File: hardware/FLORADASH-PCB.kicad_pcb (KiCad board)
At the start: 4 copper layers, 141.4 x 50.8 mm, 96 parts, among them IC1 LM66200DRLR, J1 USB_C_Receptacle_USB2.0_16P, J2 Conn_01x04_Pin, J3 Conn_02x04_Top_Bottom, Q1 FS8205, Q2 FS8205, SW1 SW_Push, SW2 SW_Push, U1 TP4056-42-ESOP8, U2 USBLC6-2SC6, U3 DW01A, U4 MT3420SP, U5 MAX17048G_T10, U6 DHT11, U7 CY8CMBR3102, U8 ESP32-C3-WROOM-02, U9 USBLC6-2SC6

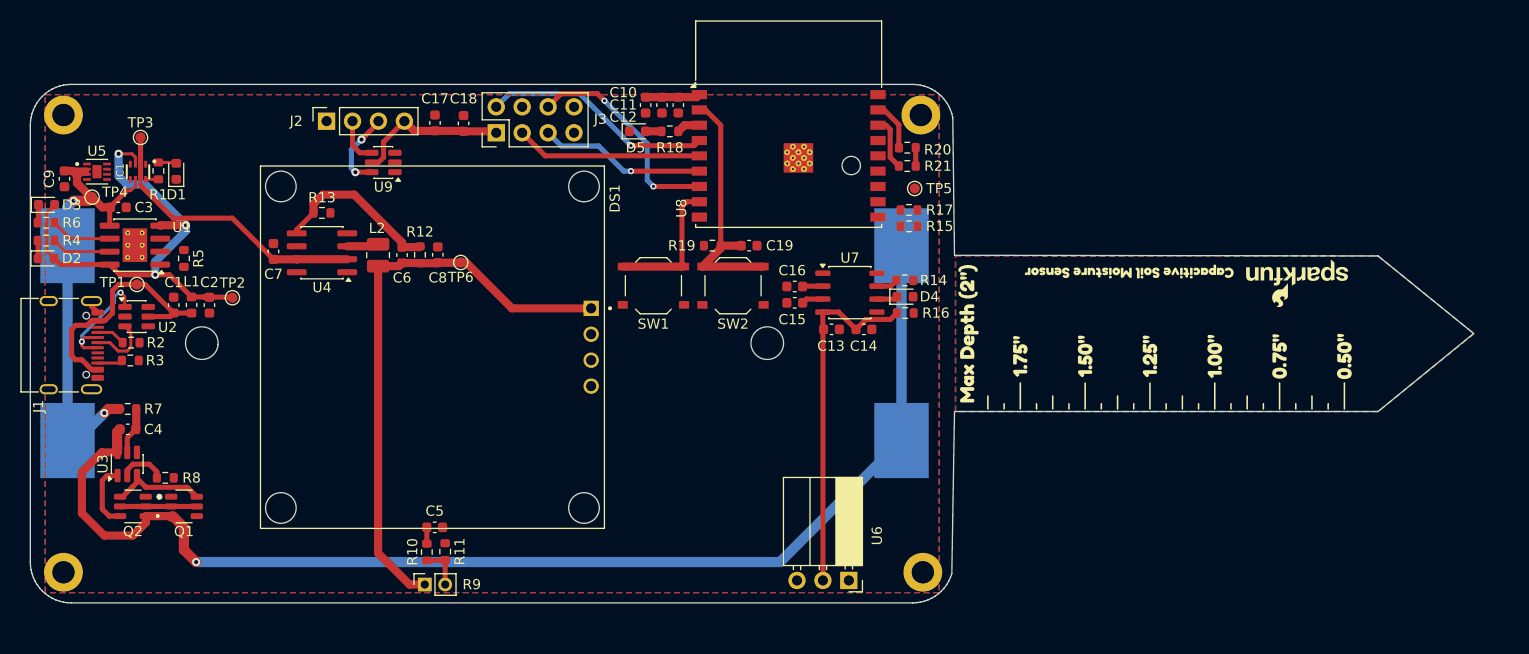
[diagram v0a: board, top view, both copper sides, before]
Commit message: Routing PCB v2
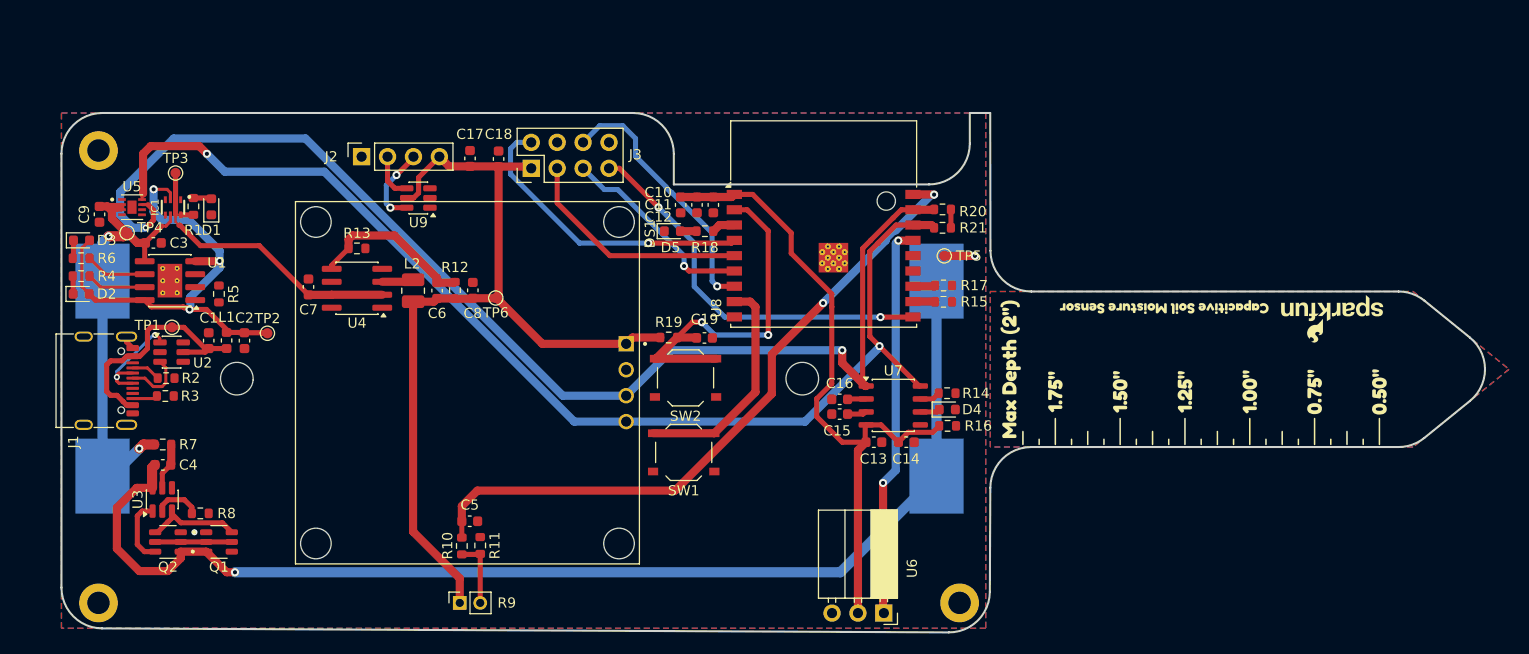
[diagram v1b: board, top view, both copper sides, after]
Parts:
- removed the G*** at (225.1, 103.8)
- removed the G*** at (225.1, 115.5)
- removed H3: MountingHole, MountingHole:MountingHole_2.2mm_M2_DIN965_Pad
- removed the kibuzzard-693B565E at (208.6, 103.5)
- removed the kibuzzard-693B565E at (208.6, 115.7)
- added G***: LOGO, SparkFun-Aesthetic:SparkFun_Logo_10mm, F.Cu at (228.6, 107.3)
- added G***: LOGO, SparkFun-Aesthetic:SparkFun_Logo_10mm, B.Cu at (228.6, 119.0)
- added kibuzzard-693B565E: G***, kibuzzard-693B565E, F.Cu at (212.0, 107.0)
- added kibuzzard-693B565E: G***, kibuzzard-693B565E, B.Cu at (212.0, 119.2)
- moved SW1 16.6 mm to (165.0, 121.3)
- moved C16 11.9 mm to (180.2, 116.1)
- moved U7 11.8 mm to (185.5, 116.7)
- moved D4 11.8 mm to (190.8, 117.1)
- moved R16 11.8 mm to (190.8, 118.7)
- moved C13 11.8 mm to (183.6, 120.3)
- moved C14 11.8 mm to (186.8, 120.3)
- moved R14 11.8 mm to (190.8, 115.5)
- moved C15 11.8 mm to (180.2, 117.5)
- moved C10 10.4 mm to (167.9, 97.0)
- moved C11 10.4 mm to (166.3, 97.0)
- moved U8 10.4 mm to (178.7, 102.0)
- moved C12 10.4 mm to (164.7, 97.0)
- moved D5 10.4 mm to (163.9, 99.6)
- moved R18 10.4 mm to (167.0, 99.6)
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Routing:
- net SCL: track 4.90 -> 120.6 mm, vias 0 -> 2
- net SDA: track 5.32 -> 114.1 mm, vias 0 -> 2
- net ADC_LUX: track 1.60 -> 66.4 mm, vias 0 -> 2
- net +3.3V: track 114.2 -> 153.9 mm
- net TEMP/HUM: track 0.00 -> 38.6 mm, vias 0 -> 2
- net GPIO10: track 0.00 -> 38.3 mm, vias 0 -> 2
- net RST: track 25.3 -> 35.4 mm, vias 0 -> 2
- net BOOT: track 13.9 -> 22.3 mm
- net GPIO5: track 22.8 -> 29.6 mm
- net GPIO8: track 21.2 -> 25.8 mm, vias 2 -> 1
- net GPIO6: track 18.3 -> 22.9 mm
- net Bat-: track 120.2 -> 124.7 mm, vias 1 -> 2
- net GPIO7: track 16.4 -> 19.6 mm
- net Net-(R10-Pad2): track 4.22 -> 6.62 mm
- net Net-(U8-IO21/TXD): track 0.00 -> 2.20 mm
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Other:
- board size 141.4 x 50.8 mm -> 139.5 x 50.9 mm
